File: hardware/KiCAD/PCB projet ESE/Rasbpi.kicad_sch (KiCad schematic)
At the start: 6 parts, among them J26 USB_C_Receptacle_USB2.0_16P, U5 USBLC6-2SC6

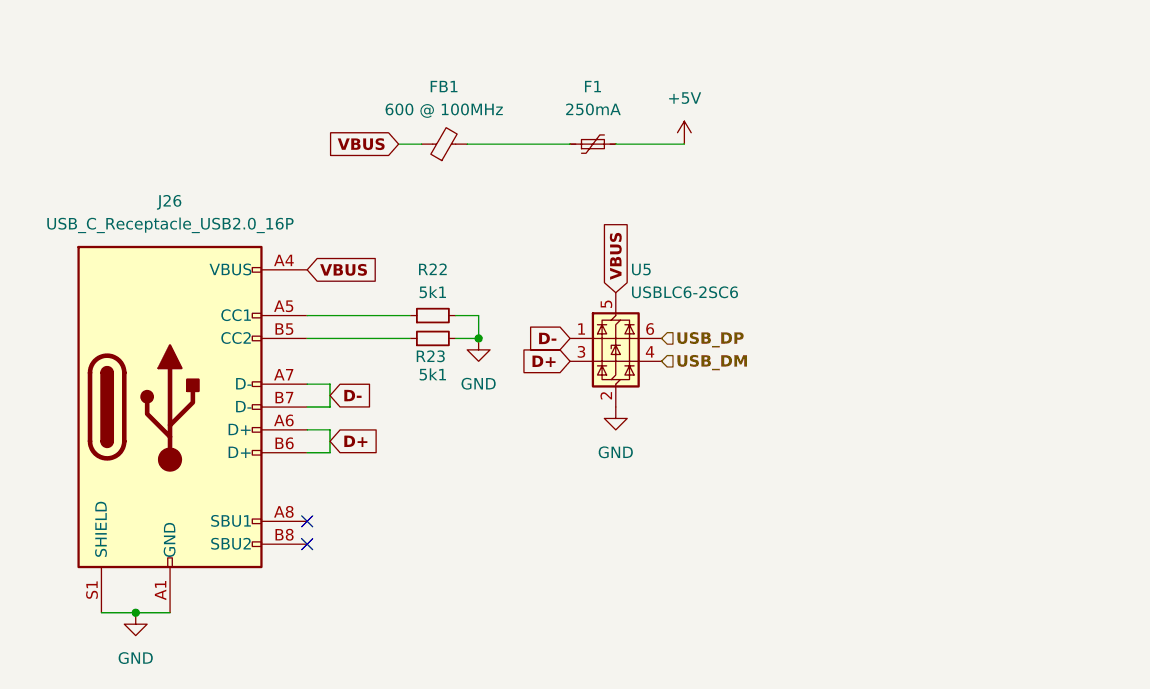
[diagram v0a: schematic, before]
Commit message: maj
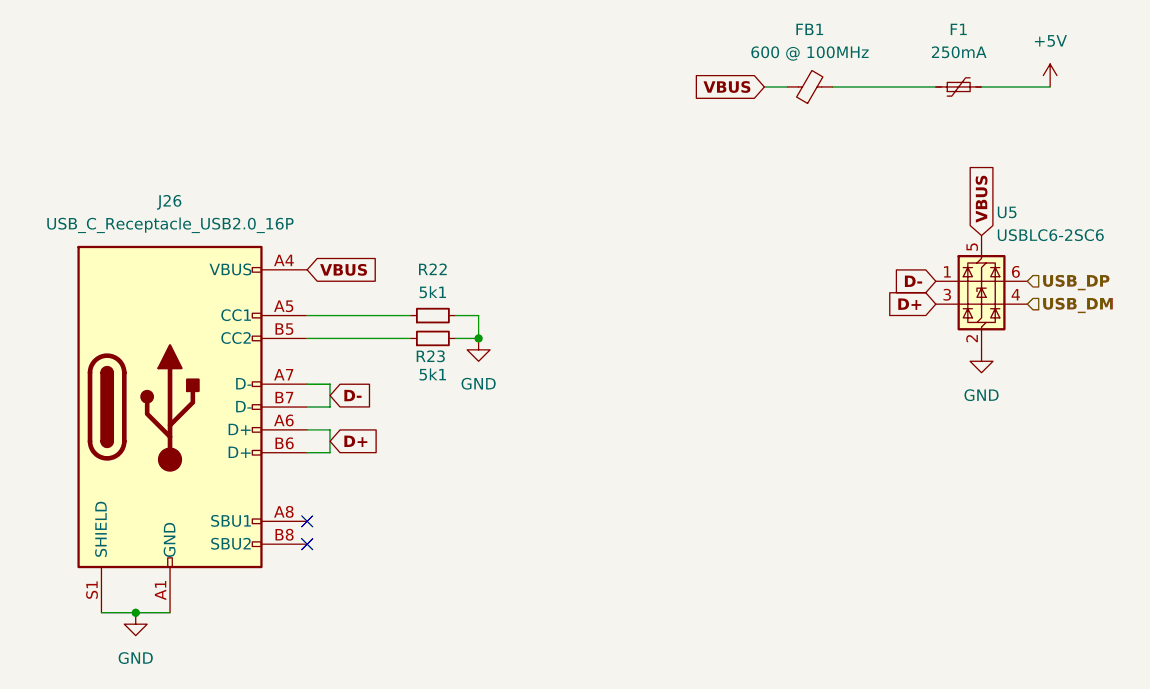
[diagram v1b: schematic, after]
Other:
- moved on the sheet: F1, FB1, U5
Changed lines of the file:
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@@
 	(wire
 		(pts
-			(xy 123.19 63.5) (xy 134.62 63.5)
+			(xy 163.83 57.15) (xy 175.26 57.15)
 		)
 		(stroke
@@
 	(wire
 		(pts
-			(xy 147.32 63.5) (xy 139.7 63.5)
+			(xy 187.96 57.15) (xy 180.34 57.15)
 		)
 		(stroke
@@
 	(wire
 		(pts
-			(xy 118.11 63.5) (xy 115.57 63.5)
+			(xy 158.75 57.15) (xy 156.21 57.15)
 		)
 		(stroke
@@
 	(global_label "VBUS"
 		(shape input)
-		(at 115.57 63.5 180)
+		(at 156.21 57.15 180)
 		(fields_autoplaced yes)
 		(effects
@@
 		)
 		(property "Intersheetrefs" "${INTERSHEET_REFS}"
-			(at 107.2102 63.5 0)
+			(at 147.8502 57.15 0)
 			(effects
 				(font
@@
 	(global_label "D+"
 		(shape input)
-		(at 134.62 87.63 180)
+		(at 175.26 81.28 180)
 		(fields_autoplaced yes)
 		(effects
@@
 		)
 		(property "Intersheetrefs" "${INTERSHEET_REFS}"
-			(at 128.3164 87.63 0)
+			(at 168.9564 81.28 0)
 			(effects
 				(font
@@
 	(global_label "VBUS"
 		(shape input)
-		(at 139.7 80.01 90)
+		(at 180.34 73.66 90)
 		(fields_autoplaced yes)
 		(effects
@@
 		)
 		(property "Intersheetrefs" "${INTERSHEET_REFS}"
-			(at 139.7 71.6502 90)
+			(at 180.34 65.3002 90)
 			(effects
 				(font
@@
 	(global_label "D-"
 		(shape input)
-		(at 134.62 85.09 180)
+		(at 175.26 78.74 180)
 		(fields_autoplaced yes)
 		(effects
@@
 		)
 		(property "Intersheetrefs" "${INTERSHEET_REFS}"
-			(at 128.3164 85.09 0)
+			(at 168.9564 78.74 0)
 			(effects
 				(font
@@
 	(hierarchical_label "USB_DM"
 		(shape input)
-		(at 144.78 87.63 0)
+		(at 185.42 81.28 0)
 		(effects
 			(font
@@
 	(hierarchical_label "USB_DP"
 		(shape input)
-		(at 144.78 85.09 0)
+		(at 185.42 78.74 0)
 		(effects
 			(font
@@
 	(symbol
 		(lib_id "power:+5V")
-		(at 147.32 63.5 0)
+		(at 187.96 57.15 0)
 		(unit 1)
 		(exclude_from_sim no)
@@
 		(fields_autoplaced yes)
 		(property "Reference" "#PWR0108"
-			(at 147.32 67.31 0)
+			(at 187.96 60.96 0)
 			(effects
 				(font
@@
 		)
 		(property "Value" "+5V"
-			(at 147.32 58.42 0)
+			(at 187.96 52.07 0)
 			(effects
 				(font
@@
 		)
 		(property "Footprint" ""
-			(at 147.32 63.5 0)
+			(at 187.96 57.15 0)
 			(effects
 				(font
@@
 		)
 		(property "Datasheet" ""
-			(at 147.32 63.5 0)
+			(at 187.96 57.15 0)
 			(effects
 				(font
@@
 		)
 		(property "Description" "Power symbol creates a global label with name \"+5V\""
-			(at 147.32 63.5 0)
+			(at 187.96 57.15 0)
 			(effects
 				(font
@@
 	(symbol
 		(lib_id "Device:FerriteBead_Small")
-		(at 120.65 63.5 90)
+		(at 161.29 57.15 90)
 		(unit 1)
 		(exclude_from_sim no)
@@
 		(fields_autoplaced yes)
 		(property "Reference" "FB1"
-			(at 120.6119 57.15 90)
+			(at 161.2519 50.8 90)
 			(effects
 				(font
@@
 		)
 		(property "Value" "600 @ 100MHz"
-			(at 120.6119 59.69 90)
+			(at 161.2519 53.34 90)
 			(effects
 				(font
@@
 		)
 		(property "Footprint" "Inductor_SMD:L_0805_2012Metric"
-			(at 120.65 65.278 90)
+			(at 161.29 58.928 90)
 			(effects
 				(font
@@
 		)
 		(property "Datasheet" "~"
-			(at 120.65 63.5 0)
+			(at 161.29 57.15 0)
 			(effects
 				(font
@@
 		)
 		(property "Description" "Ferrite bead, small symbol"
-			(at 120.65 63.5 0)
+			(at 161.29 57.15 0)
 			(effects
 				(font
@@
 	(symbol
 		(lib_id "Device:Polyfuse_Small")
-		(at 137.16 63.5 90)
+		(at 177.8 57.15 90)
 		(unit 1)
 		(exclude_from_sim no)
@@
 		(fields_autoplaced yes)
 		(property "Reference" "F1"
-			(at 137.16 57.15 90)
+			(at 177.8 50.8 90)
 			(effects
 				(font
@@
 		)
 		(property "Value" "250mA"
-			(at 137.16 59.69 90)
+			(at 177.8 53.34 90)
 			(effects
 				(font
@@
 		)
 		(property "Footprint" "Fuse:Fuse_1206_3216Metric"
-			(at 142.24 62.23 0)
+			(at 182.88 55.88 0)
 			(effects
 				(font
@@
 		)
 		(property "Datasheet" "~"
-			(at 137.16 63.5 0)
+			(at 177.8 57.15 0)
 			(effects
 				(font
@@
 		)
 		(property "Description" "Resettable fuse, polymeric positive temperature coefficient, small symbol"
-			(at 137.16 63.5 0)
+			(at 177.8 57.15 0)
 			(effects
 				(font
@@
 	(symbol
 		(lib_id "power:GND")
-		(at 139.7 92.71 0)
+		(at 180.34 86.36 0)
 		(unit 1)
 		(exclude_from_sim no)
@@
 		(fields_autoplaced yes)
 		(property "Reference" "#PWR0107"
-			(at 139.7 99.06 0)
+			(at 180.34 92.71 0)
 			(effects
 				(font
@@
 		)
 		(property "Value" "GND"
-			(at 139.7 97.79 0)
+			(at 180.34 91.44 0)
 			(effects
 				(font
@@
 		)
 		(property "Footprint" ""
-			(at 139.7 92.71 0)
+			(at 180.34 86.36 0)
 			(effects
 				(font
@@
 		)
 		(property "Datasheet" ""
-			(at 139.7 92.71 0)
+			(at 180.34 86.36 0)
 			(effects
 				(font
@@
 		)
 		(property "Description" "Power symbol creates a global label with name \"GND\" , ground"
-			(at 139.7 92.71 0)
+			(at 180.34 86.36 0)
 			(effects
 				(font
@@
 	(symbol
 		(lib_id "Power_Protection:USBLC6-2SC6")
-		(at 139.7 85.09 0)
+		(at 180.34 78.74 0)
 		(unit 1)
 		(exclude_from_sim no)
@@
 		(fields_autoplaced yes)
 		(property "Reference" "U5"
-			(at 141.3511 77.47 0)
+			(at 181.9911 71.12 0)
 			(effects
 				(font
@@
 		)
 		(property "Value" "USBLC6-2SC6"
-			(at 141.3511 80.01 0)
+			(at 181.9911 73.66 0)
 			(effects
 				(font
@@
 		)
 		(property "Footprint" "Package_TO_SOT_SMD:SOT-23-6"
-			(at 140.97 91.44 0)
+			(at 181.61 85.09 0)
 			(effects
 				(font
@@
 		)
 		(property "Datasheet" "https://www.st.com/resource/en/datasheet/usblc6-2.pdf"
-			(at 140.97 93.345 0)
+			(at 181.61 86.995 0)
 			(effects
 				(font
@@
 		)
 		(property "Description" "Very low capacitance ESD protection diode, 2 data-line, SOT-23-6"
-			(at 139.7 85.09 0)
+			(at 180.34 78.74 0)
 			(effects
 				(font
@@
 		)
 		(property "MPN" "624-7693"
-			(at 139.7 85.09 0)
-			(effects
-				(font
+			(at 180.34 78.74 0)
+			(effects
+				(font
